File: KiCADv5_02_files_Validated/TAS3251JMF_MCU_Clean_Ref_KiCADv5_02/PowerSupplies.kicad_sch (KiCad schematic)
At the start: 53 parts, among them IC1 LM5010MHX, J18 Conn_01x04, J5 PVDD, J6 Conn_01x01_Male, J7 Conn_01x01_Male, J8 Conn_01x01_Male, J9 Conn_01x01_Male, U2 AMS1117-3.3, U3 LM2940-12

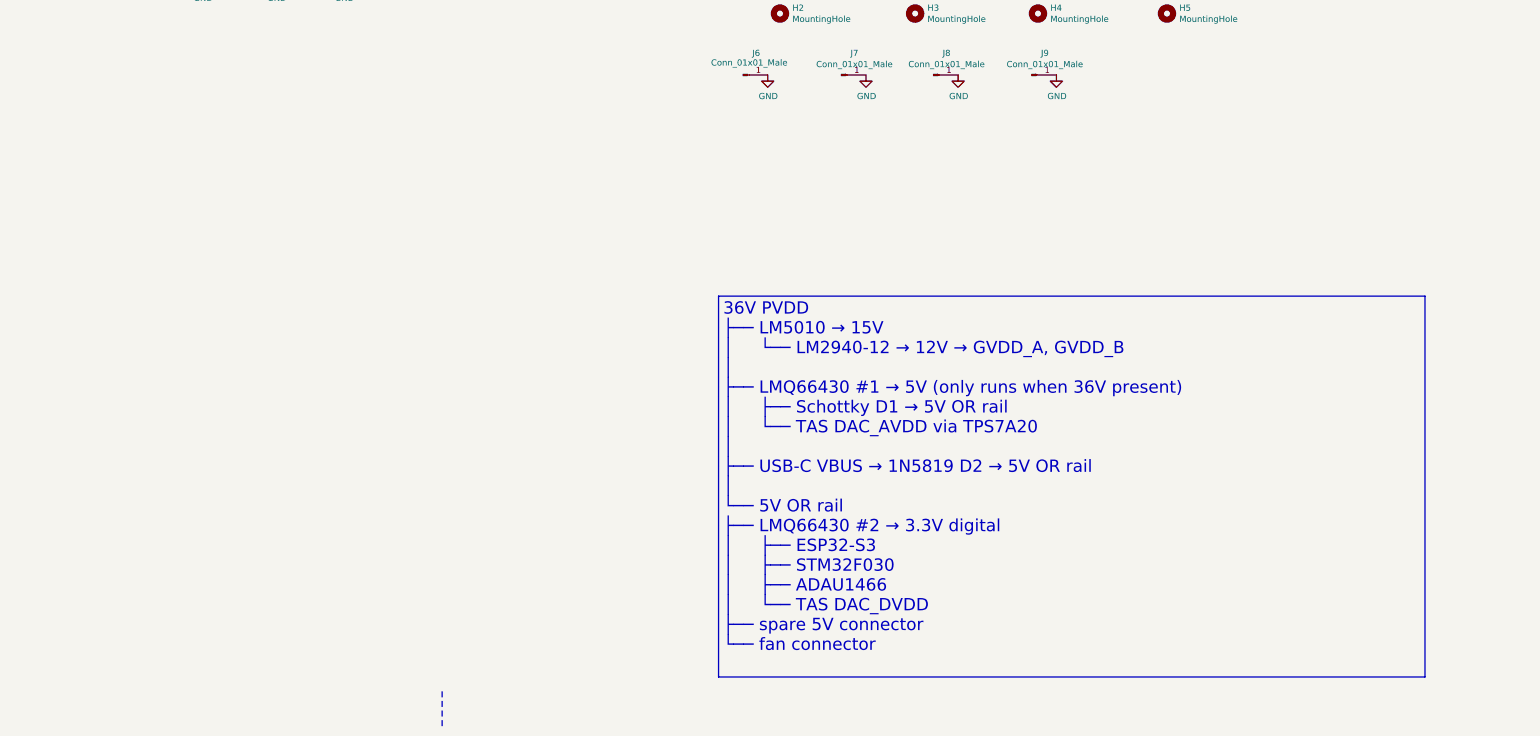
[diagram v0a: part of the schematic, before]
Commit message: Adding PS
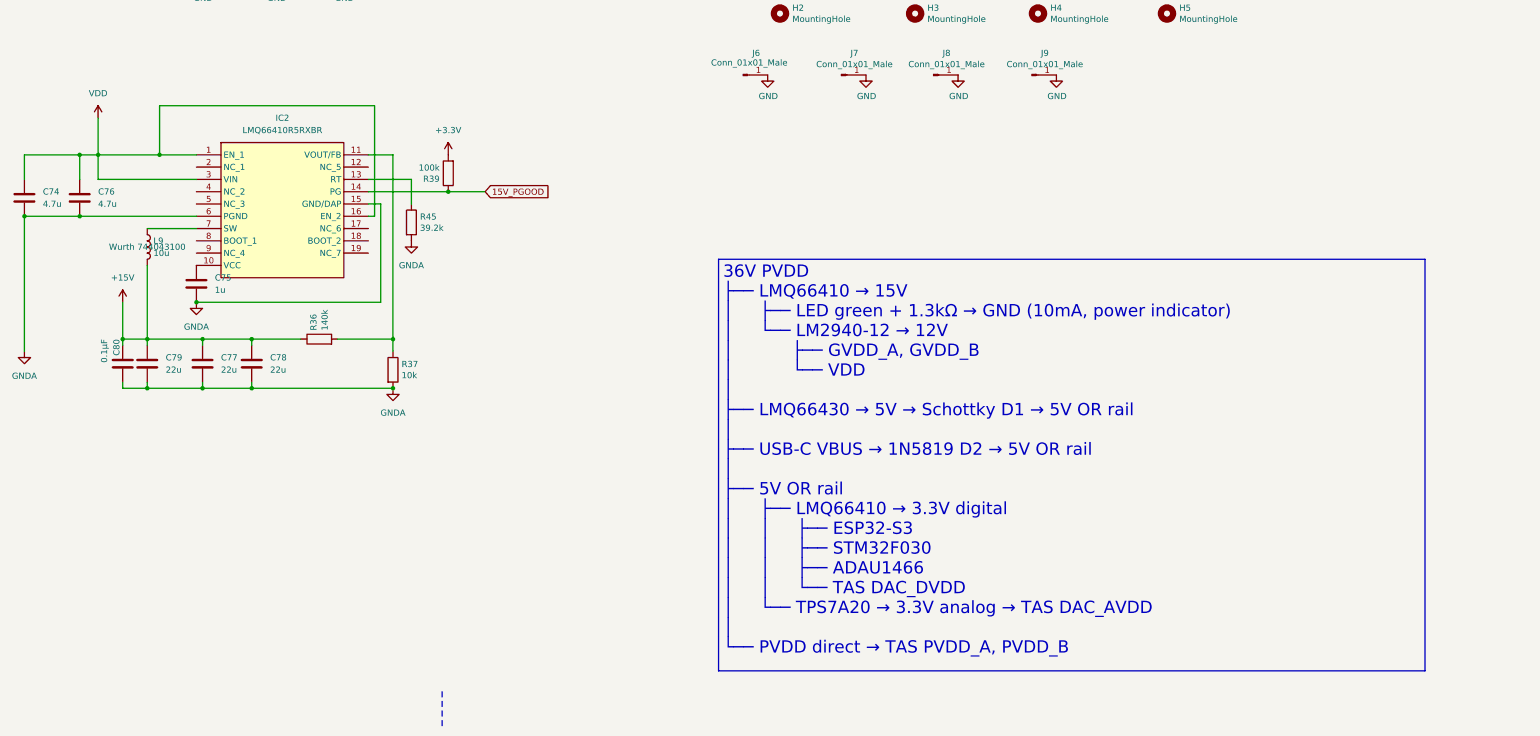
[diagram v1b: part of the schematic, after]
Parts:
- added C74, C76: 4.7u, Capacitor_SMD:C_1812_4532Metric_Pad1.57x3.40mm_HandSolder, symbol Device:C
- added C75: 1u, Capacitor_SMD:C_0805_2012Metric_Pad1.18x1.45mm_HandSolder, symbol Device:C
- added C77, C78, C79: 22u, Capacitor_SMD:C_1812_4532Metric_Pad1.57x3.40mm_HandSolder, symbol Device:C
- added C80: 0.1µF, Capacitor_SMD:C_0805_2012Metric_Pad1.15x1.40mm_HandSolder, symbol Device:C
- added IC2: LMQ66410R5RXBR, TAS3251:LMR66430R5RXBR, symbol LMQ66430R5RXBR:LMQ66410R5RXBR
- added L9: 10u, Inductor_SMD:L_Wuerth_LQFS-4828, symbol Device:L
- added R36: 140k, Resistor_SMD:R_0805_2012Metric_Pad1.15x1.40mm_HandSolder, symbol Device:R
- added R37: 10k, Resistor_SMD:R_0805_2012Metric_Pad1.15x1.40mm_HandSolder, symbol Device:R
- added R39: 100k, Resistor_SMD:R_0805_2012Metric_Pad1.15x1.40mm_HandSolder, symbol Device:R
- added R45: 39.2k, Resistor_SMD:R_0805_2012Metric_Pad1.15x1.40mm_HandSolder, symbol Device:R
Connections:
- net +15V: now also C77.1, C78.1, C79.1, C80.2, L9.2, R36.1
- net +3.3V: now also R39.2
- net VDD: now also C74.1, C76.1, IC2.1 (EN_1), IC2.16 (EN_2), IC2.3 (VIN)
- new net: IC2.11 (VOUT/FB), R36.2, R37.1
- new net: IC2.7 (SW), L9.1
- new net: IC2.13 (RT), R45.1
- new net: C75.1, IC2.10 (VCC)
- new net 15V_PGOOD: IC2.14 (PG), R39.1
- new net GNDA: C74.2, C75.2, C76.2, C77.2, C78.2, C79.2, C80.1, IC2.15 (GND/DAP), IC2.6 (PGND), R37.2, R45.2

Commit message: modified PSU
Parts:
- removed C59, C60: 2.2µF, Capacitor_SMD:C_1206_3216Metric_Pad1.42x1.75mm_HandSolder, symbol Device:C
- removed C61: 4.7µF, Capacitor_SMD:C_1206_3216Metric_Pad1.42x1.75mm_HandSolder, symbol Device:C
- removed D3: D_Schottky, Diode_SMD:D_SOD-123F, symbol Device:D_Schottky
- removed IC1: LM5010MHX, SamacSys_Parts:SOP65P640X110-15N, symbol TAS3251JMF_MCU-rescue:LM5010AMH-SamacSys_Parts
- removed JP5: Jumper_2_Bridged, Connector_PinHeader_2.54mm:PinHeader_1x02_P2.54mm_Vertical, symbol Jumper:Jumper_2_Bridged
- removed L5: 150µH, TAS3251:L_Wuerth_74404064151_Handsolder, symbol Device:L
- removed R44: NoPOP, Resistor_SMD:R_0603_1608Metric_Pad1.05x0.95mm_HandSolder, symbol Device:R
- added IC1: LMQ66410R5RXBR, TAS3251:LMR66430R5RXBR, symbol LMQ66430R5RXBR:LMQ66410R5RXBR
- added L10: 10u, Inductor_SMD:L_Wuerth_LQFS-4828, symbol Device:L
- C44: value 2.2µF -> 4.7u; footprint Capacitor_SMD:C_1206_3216Metric_Pad1.42x1.75mm_HandSolder -> Capacitor_SMD:C_1812_4532Metric_Pad1.57x3.40mm_HandSolder; Manufacturer TDK -> (none); Manufacturer_Name CL31B225KBHNNNE -> (none); Manufacturer_Part_Number C50254 -> (none); PartNumber NOPOP -> (none)
- C45: value 0.1µF -> 4.7u; footprint Capacitor_SMD:C_0805_2012Metric_Pad1.15x1.40mm_HandSolder -> Capacitor_SMD:C_1812_4532Metric_Pad1.57x3.40mm_HandSolder; Manufacturer YAGEO -> (none); Manufacturer_Part_Number C49678 -> (none); PartNumber CC0805KRX7R9BB104 -> (none); Value2 x50V -> (none); ValueDisplayed 0.1µF -> (none)
- C46: value 4700pF -> 0.1µF; Manufacturer YAGEO -> (none); Manufacturer_Name 0805B472K500NT -> (none); Manufacturer_Part_Number C1744 -> C49678; PartNumber CC0805KRX7R9BB472 -> (none); Value2 x50V -> x25V
- C48: value 0.47µF -> 22u; footprint Capacitor_SMD:C_0805_2012Metric_Pad1.15x1.40mm_HandSolder -> Capacitor_SMD:C_1812_4532Metric_Pad1.57x3.40mm_HandSolder; Manufacturer_Name CL21B474KBFNNNE -> (none); Manufacturer_Part_Number C13967 -> (none); Value2 x50V -> (none)
- C49: value 0.1µF -> 1u; footprint Capacitor_SMD:C_0805_2012Metric_Pad1.15x1.40mm_HandSolder -> Capacitor_SMD:C_0805_2012Metric_Pad1.18x1.45mm_HandSolder; Manufacturer_Part_Number C49678 -> (none); Value2 x25V -> (none)
- C50: value 4700pF -> 22u; footprint Capacitor_SMD:C_0805_2012Metric_Pad1.15x1.40mm_HandSolder -> Capacitor_SMD:C_1812_4532Metric_Pad1.57x3.40mm_HandSolder; Manufacturer Guangdong Fenghua Advanced Tech -> (none); Manufacturer_Name 0805B472K500NT -> (none); Manufacturer_Part_Number C1744 -> (none); PartNumber C1744 -> (none); Value2 x50V -> (none)
- C52: value 4.7µF -> 22u; footprint Capacitor_SMD:C_1206_3216Metric_Pad1.42x1.75mm_HandSolder -> Capacitor_SMD:C_1812_4532Metric_Pad1.57x3.40mm_HandSolder; Manufacturer Murata -> (none); Manufacturer_Name 1206B475K500NT -> (none); Manufacturer_Part_Number C29823 -> (none); PartNumber GRM31CR71H475KA12L -> (none)
- R18: value 1.02k -> 10k; Manufacturer YAGEO -> (none); Manufacturer_Part_Number C17513 -> (none); PartNumber RC0805FR-071KL -> (none); ValueDisplayed 1k -> (none)
- R19: value 365k -> 39.2k; Manufacturer UniRoyql Elec -> (none); Manufacturer_Part_Number C25825 -> (none); PartNumber C17647 -> (none); ValueDisplayed 365k -> (none)
- R38: value 0 -> 100k; footprint Resistor_SMD:R_0603_1608Metric_Pad1.05x0.95mm_HandSolder -> Resistor_SMD:R_0805_2012Metric_Pad1.15x1.40mm_HandSolder; Manufacturer_Name 0603WAF0000T5E -> (none); Manufacturer_Part_Number C21189 -> (none)
- R7: value 5.1k -> 140k; Manufacturer 0805W8F5101T5E -> (none); Manufacturer_Part_Number C27834 -> (none); PartNumber C27834 -> (none)
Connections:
- net +15V: no longer C50.1, C52.1, R7.1
- net +3.3V: now also R38.2
- net GND: no longer C44.2, C45.2, C46.2, C48.1, R18.2, R38.2
- net GNDA: now also C44.2, C45.2, C46.1, C48.2, C49.2, C50.2, C52.2, R18.2, R19.2, IC1.15 (GND/DAP), IC1.6 (PGND)
- net VDD: now also C44.1, C45.1, IC1.1 (EN_1), IC1.16 (EN_2), IC1.3 (VIN)
- net at C49.1: now also IC1.10 (VCC)
- net at R18.1, R7.2: now also IC1.11 (VOUT/FB); no longer C50.2
- net at R19.1: now also IC1.13 (RT)
- net 5V_PGOOD: now reaches R38.1
- net 5V_PGOOD: now also IC1.14 (PG); no longer C52.2
- new net: IC1.7 (SW), L10.1
- new net 5V: C46.2, C48.1, C50.1, C52.1, L10.2, R7.1
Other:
- note removed: "Final design of LM5010 stage as of LM5010_15V_0.5A_330kHz final decision.pdf"
- moved on the sheet: C74, C75, C76, C77, C78, C79, C80, D4, D5, H2, H3, H4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
